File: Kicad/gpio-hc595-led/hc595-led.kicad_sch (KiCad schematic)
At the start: 22 parts, among them K1 GPIO IN, K2 GPIO OUT, U1 74HC595-SOIC-16, U2 3M-SJ5376

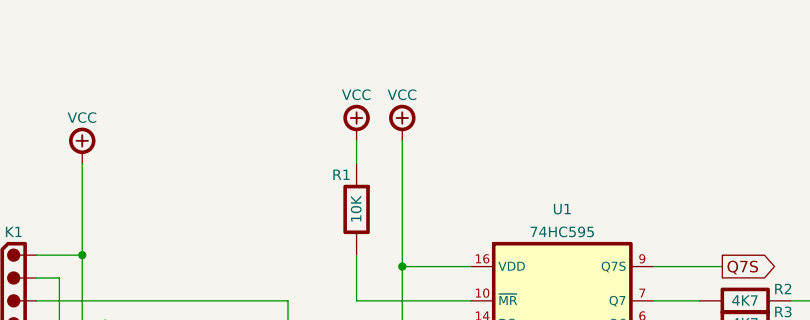
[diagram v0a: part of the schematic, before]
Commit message: Update
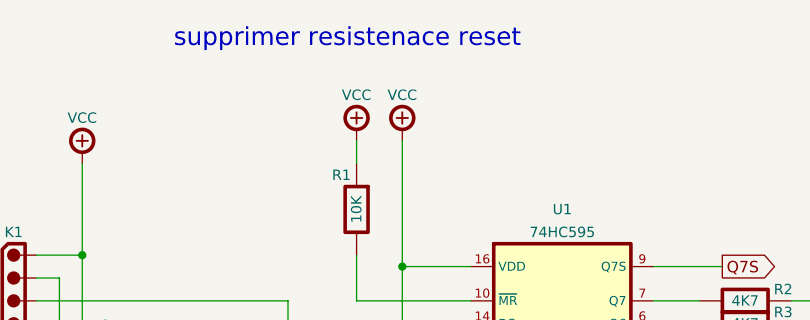
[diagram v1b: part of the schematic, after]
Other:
- note added: "supprimer resistenace reset"
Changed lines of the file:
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@@
     (effects (font (size 1.27 1.27)) (justify right bottom))
+  )
+  (text "supprimer resistenace reset" (at 106.68 53.34 0)
+    (effects (font (size 2 2)) (justify left bottom))
   )
   (text "~{OE}" (at 86.36 90.17 180)

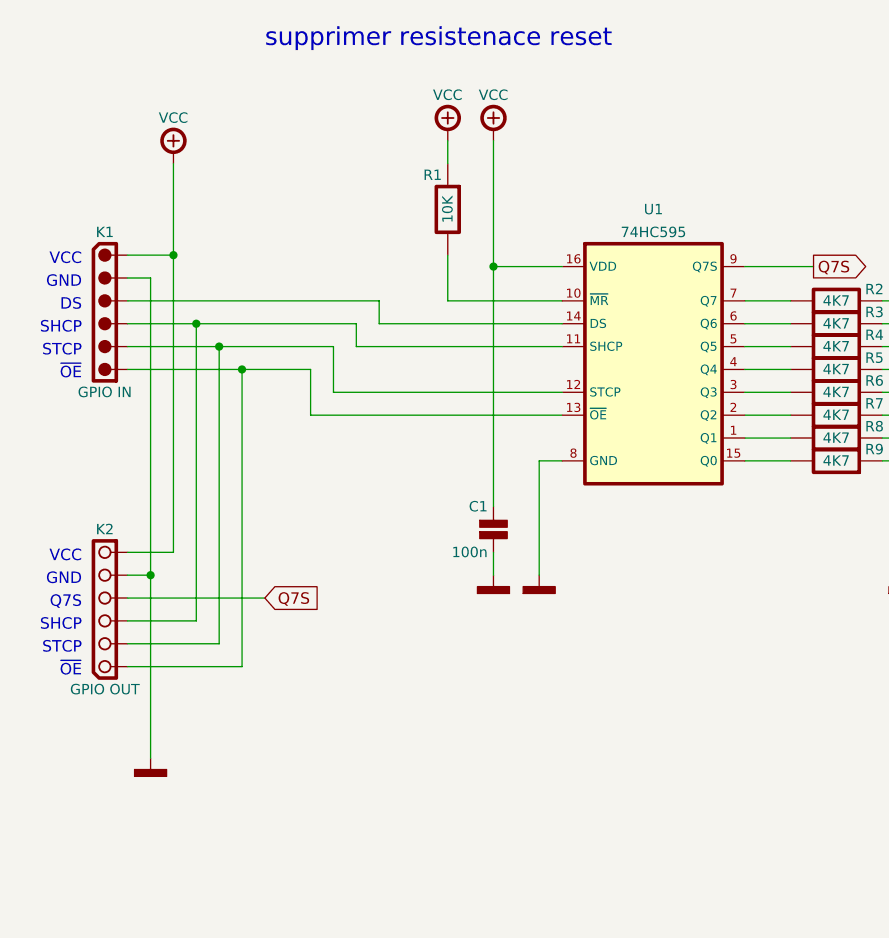
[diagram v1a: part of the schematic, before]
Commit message: Update
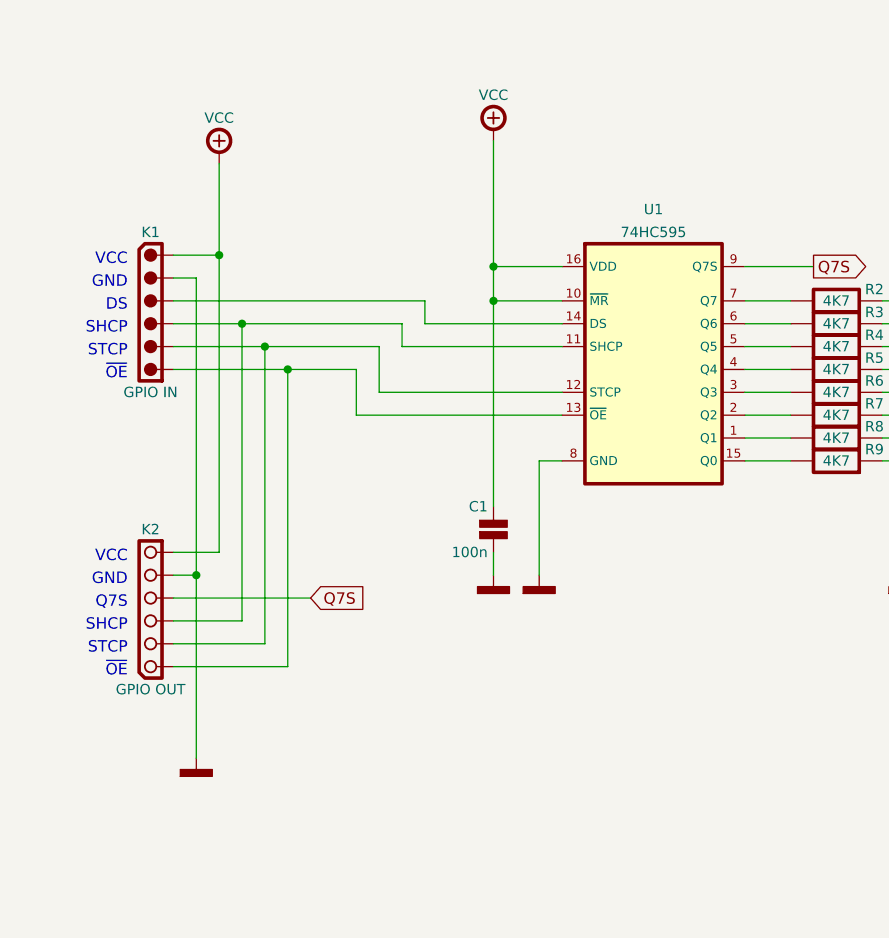
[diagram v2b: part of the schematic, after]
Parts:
- removed R1: 10K, tronixio:RESISTOR-1206, symbol tronixio:R-1210
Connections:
- net VCC: now also U1.10 (~{MR})
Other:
- note removed: "supprimer resistenace reset"
- moved on the sheet: K1, K2

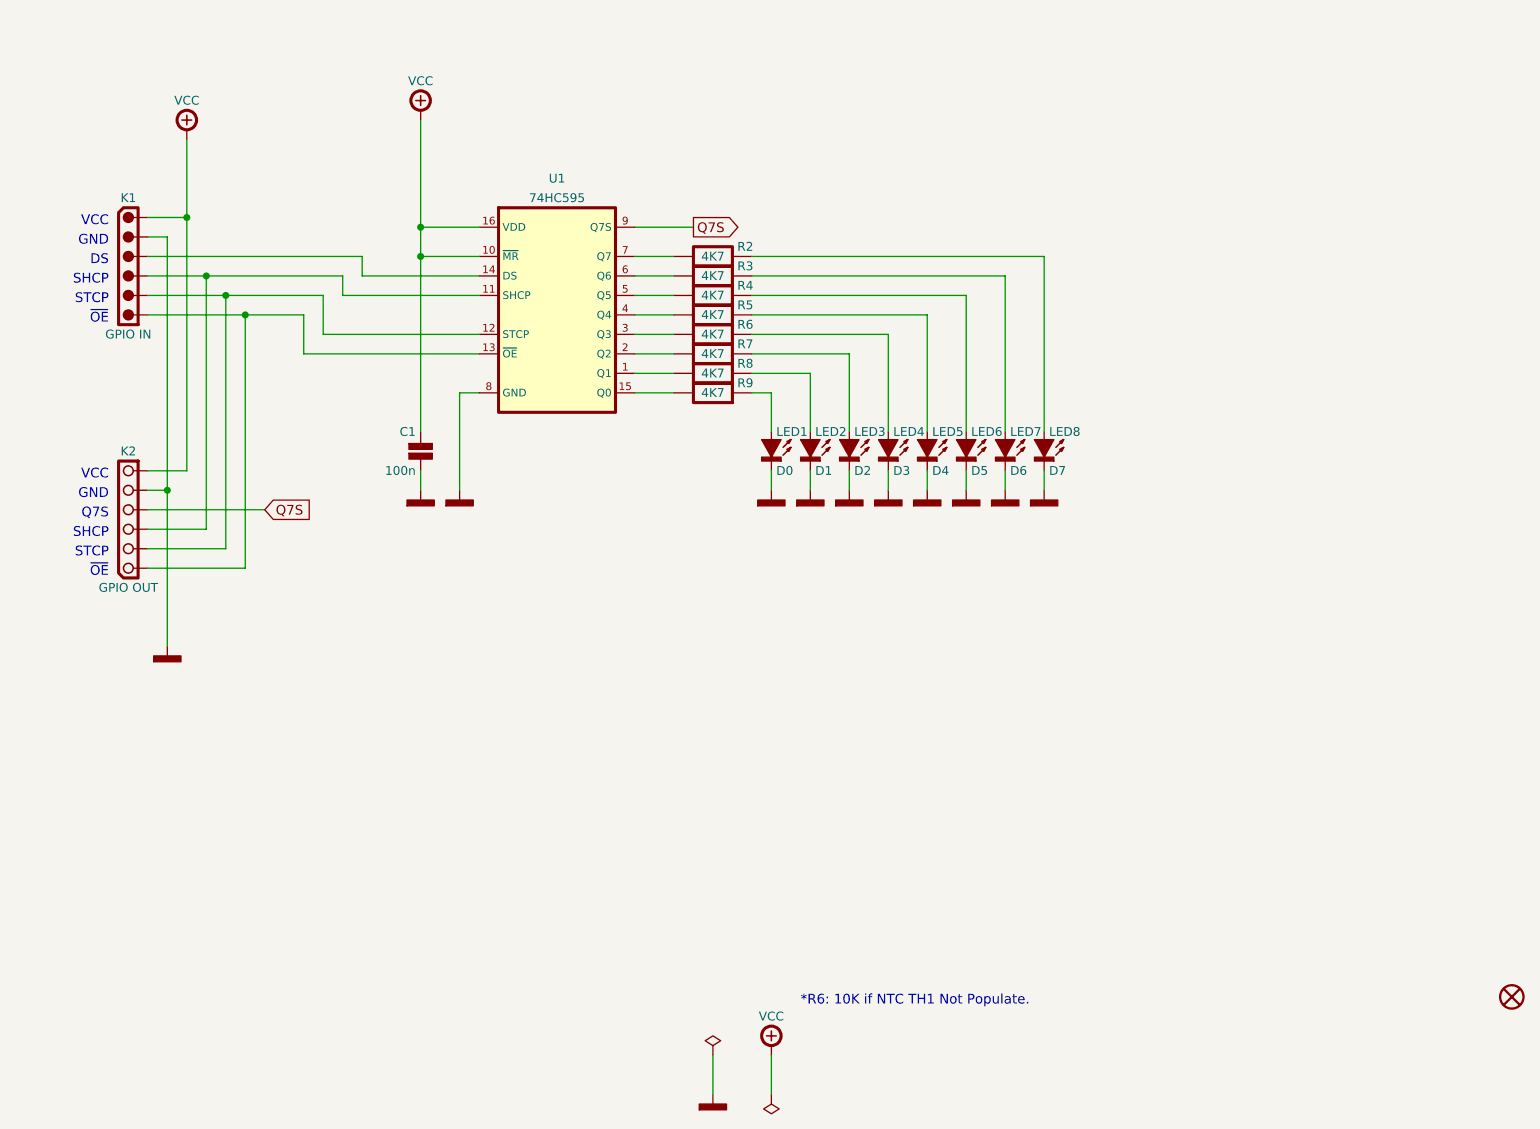
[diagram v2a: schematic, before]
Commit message: Update
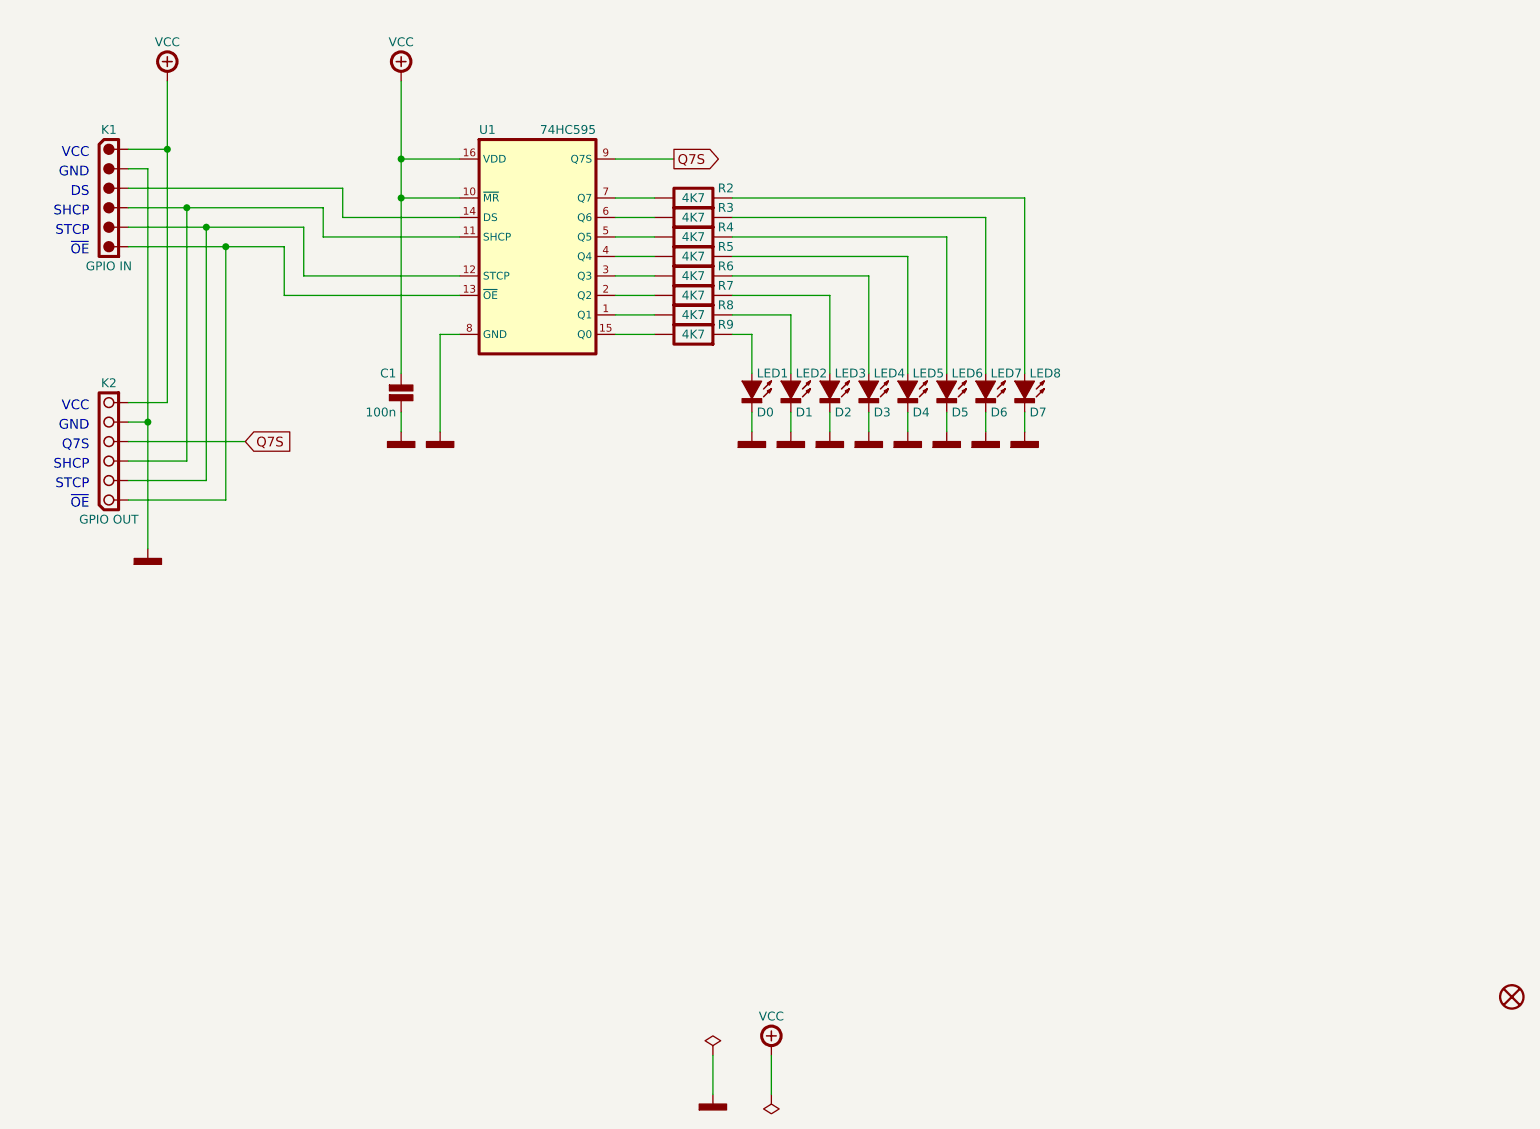
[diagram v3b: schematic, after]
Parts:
- C1: symbol tronixio:C-1206 -> tronixio:CAPACITOR; Tolerance (none) -> 20%; Voltage (none) -> 50V
- K2: Name (none) -> SAMTEC-SSW-106-02-T-S-RA
- R2, R3, R4, R5, R6, R7, R8, R9: symbol tronixio:R-1210 -> tronixio:RESISTOR; Tolerance (none) -> 5%
- U2: footprint tronixio:zzz3M-SJ5376 -> tronixio:3M-SJ5376
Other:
- note removed: "*R6: 10K if NTC TH1 Not Populate."
- moved on the sheet: C1, K1, K2, LED1, LED2, LED3, LED4, LED5, LED6, LED7, LED8, R2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

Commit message: Update
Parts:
- removed C1: 100n, tronixio:CAPACITOR-1206, symbol tronixio:CAPACITOR
- added C1: CAPACITOR-1206-100N, tronixio:CAPACITOR-1206, symbol tronixio:CAPACITOR-1206-100N
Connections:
- net GND: now also C1.2
- net VCC: now also C1.1
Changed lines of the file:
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@@
-    (pin "2")
-  )
-  (symbol (lib_id "tronixio:CAPACITOR") (at 129.54 99.06 0) (unit 1)
-    (in_bom yes) (on_board yes)
-    (property "Reference" "C1" (id 0) (at 128.905 96.52 0)
-      (effects (font (size 1.15 1.15)) (justify right))
-    )
-    (property "Value" "100n" (id 1) (at 128.905 101.6 0)
-      (effects (font (size 1.15 1.15)) (justify right))
-    )
-    (property "Footprint" "tronixio:CAPACITOR-1206" (id 2) (at 129.54 110.49 0)
-      (effects (font (size 1 1)) hide)
-    )
-    (property "Datasheet" "" (id 3) (at 129.54 101.6 0)
-      (effects (font (size 1 1)) hide)
-    )
-    (property "Voltage" "50V" (id 4) (at 129.54 107.95 0)
-      (effects (font (size 1.15 1.15)) hide)
-    )
-    (property "Tolerance" "20%" (id 5) (at 132.08 104.14 0)
-      (effects (font (size 1.15 1.15)) hide)
-    )
-    (property "Mouser" "" (id 6) (at 129.54 99.06 0)
-      (effects (font (size 1 1)) hide)
-    )
-    (pin "1")
     (pin "2")
   )
@@
     (property "Mouser" "~" (id 5) (at 187.96 83.82 0)
       (effects (font (size 1 1)) hide)
+    )
+    (pin "1")
+    (pin "2")
+  )
+  (symbol (lib_id "tronixio:CAPACITOR-1206-100N") (at 129.54 99.06 0) (unit 1)
+    (in_bom yes) (on_board yes)
+    (property "Reference" "C1" (id 0) (at 128.905 96.52 0)
+      (effects (font (size 1.15 1.15)) (justify right))
+    )
+    (property "Value" "CAPACITOR-1206-100N" (id 1) (at 129.54 109.22 0)
+      (effects (font (size 1 1)) hide)
+    )
+    (property "Footprint" "tronixio:CAPACITOR-1206" (id 2) (at 129.54 111.76 0)
+      (effects (font (size 1 1)) hide)
+    )
+    (property "Datasheet" "https://content.kemet.com/datasheets/KEM_C1090_X7R_ESD.pdf" (id 3) (at 129.54 114.3 0)
+      (effects (font (size 1 1)) hide)
+    )
+    (property "Voltage" "50V" (id 4) (at 130.175 103.505 0)
+      (effects (font (size 1.15 1.15)) (justify left) hide)
+    )
+    (property "Tolerance" "20%" (id 5) (at 130.175 105.41 0)
+      (effects (font (size 1.15 1.15)) (justify left) hide)
+    )
+    (property "Mouser" "80-C1206C104M5R" (id 6) (at 129.54 116.84 0)
+      (effects (font (size 1 1)) hide)
+    )
+    (property "Name" "100n" (id 7) (at 128.905 101.6 0)
+      (effects (font (size 1.15 1.15)) (justify right))
     )
     (pin "1")
@@
       (reference "#PWR016") (unit 1) (value "POWER-GND") (footprint "")
     )
-    (path "/1292386c-01d2-4aa5-a5bf-25821c6789db"
-      (reference "C1") (unit 1) (value "100n") (footprint "tronixio:CAPACITOR-1206")
+    (path "/92a36e64-9c6c-4d7f-812b-59a758389474"
+      (reference "C1") (unit 1) (value "CAPACITOR-1206-100N") (footprint "tronixio:CAPACITOR-1206")
     )
     (path "/9c4c3158-1d24-4d1c-8e39-342d19a63c17"
